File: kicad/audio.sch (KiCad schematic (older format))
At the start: 18 parts, among them J301 ST-214N, J302 ST-214N, J303 ST-214N, U301 AD824

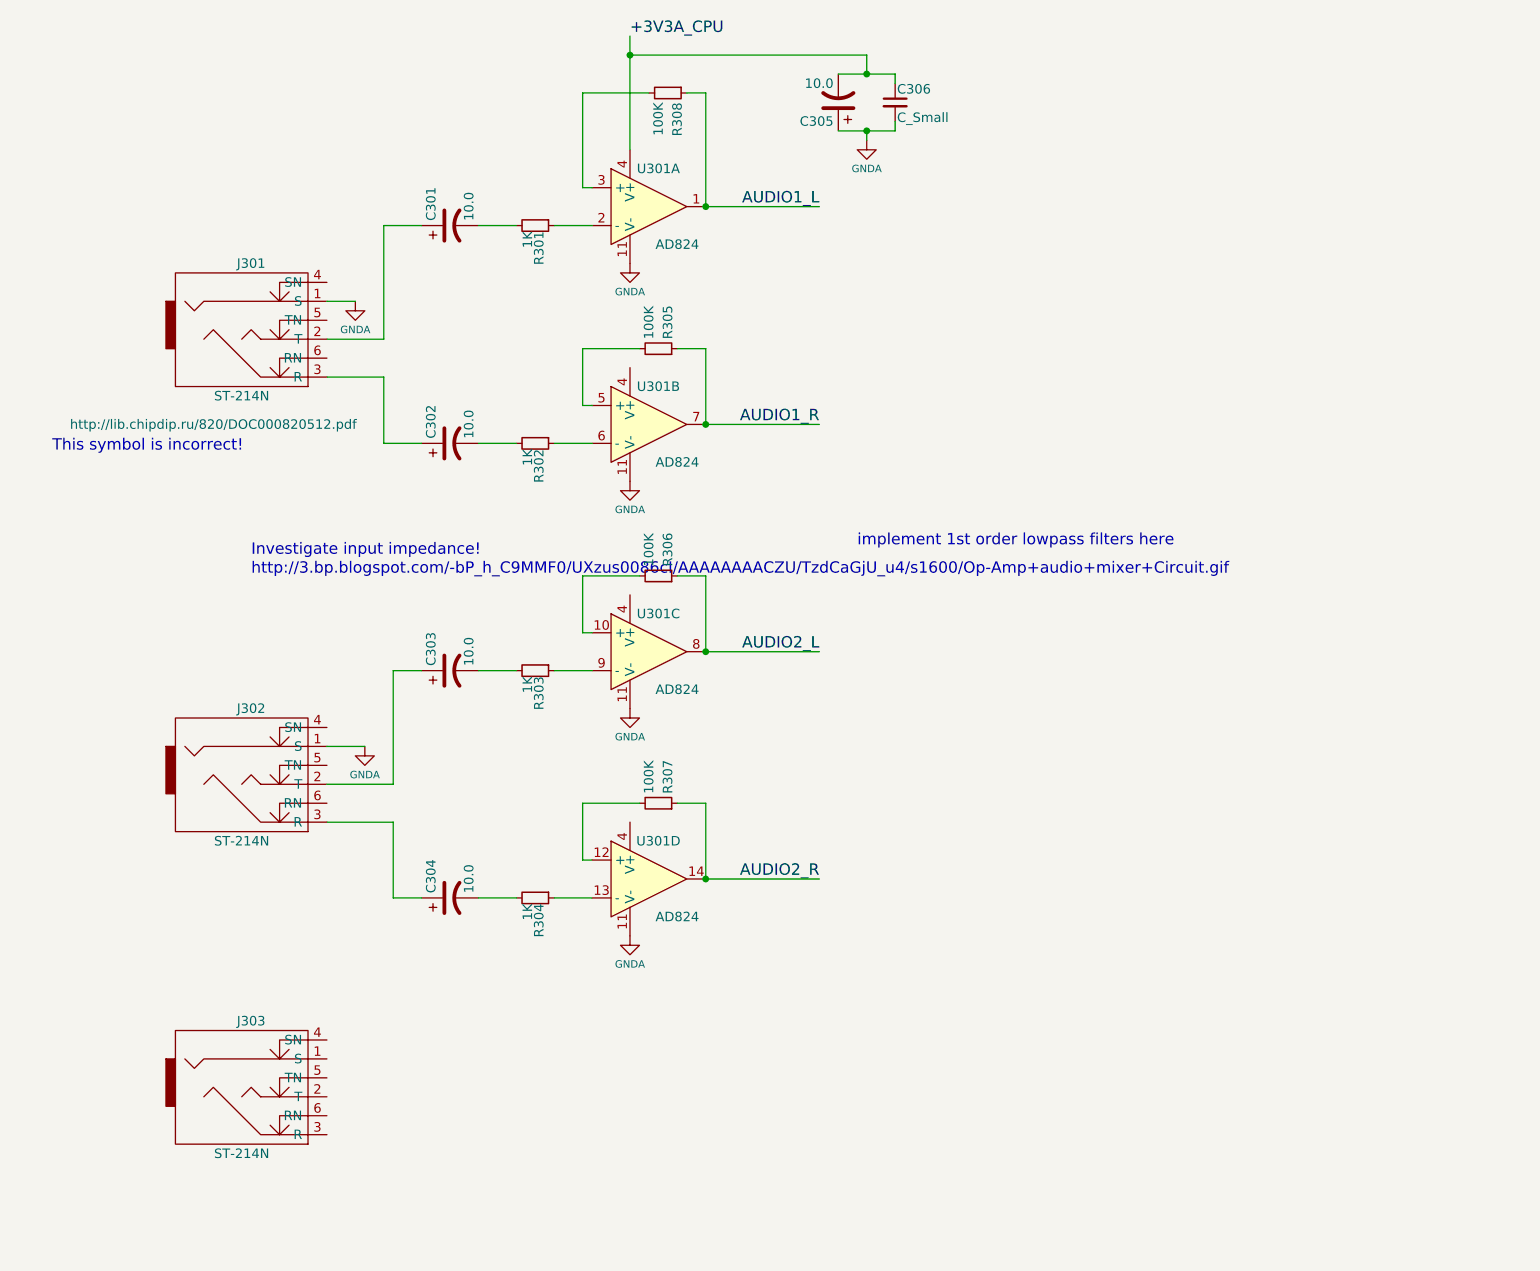
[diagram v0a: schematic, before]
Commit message: ...
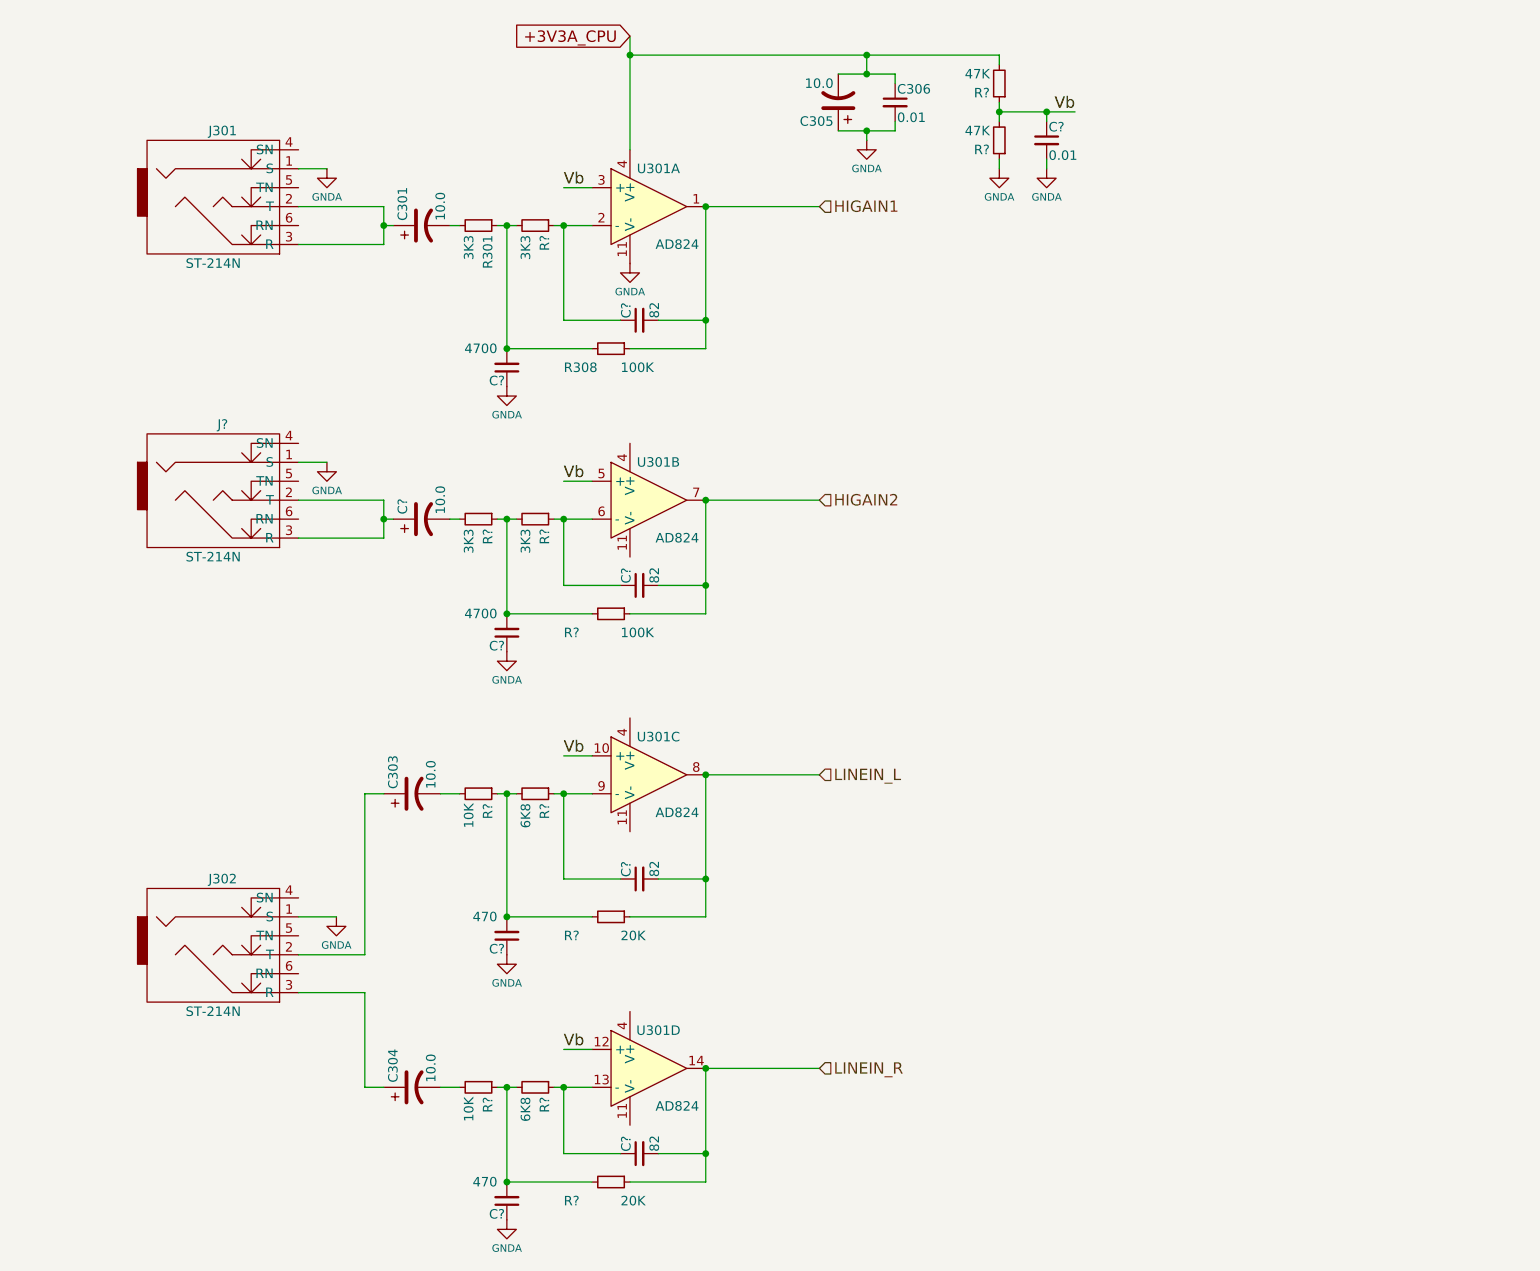
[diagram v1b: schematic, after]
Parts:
- removed C302: 10.0, symbol CP1
- removed J303: ST-214N, symbol JACK_TRS_6PINS
- removed R302, R303, R304: 1K, symbol R_Small
- removed R305, R306, R307: 100K, symbol R_Small
- added C? (x4): 82, symbol C_Small
- added C? (x2): 4700, symbol C_Small
- added C?: 0.01, symbol C_Small
- added C?: 10.0, symbol CP1
- added C? (x2): 470, symbol C_Small
- added J?: ST-214N, symbol JACK_TRS_6PINS
- added R? (x3): 3K3, symbol R_Small
- added R? (x2): 47K, symbol R_Small
- added R?: 100K, symbol R_Small
- added R? (x2): 10K, symbol R_Small
- added R? (x2): 20K, symbol R_Small
- added R? (x2): 6K8, symbol R_Small
- C306: value C_Small -> 0.01
- R301: value 1K -> 3K3
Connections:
- net +3V3A_CPU: now also R?.2
- net GNDA: now also C?.1, C?.1, C?.1, C?.1, C?.2, J?.1 (S), R?.1; no longer U301.11 (V-), U301.11 (V-), U301.11 (V-)
- net at C301.1, J301.2 (T): now also J301.3 (R)
- net at U301.2 (-): now also C?.1, R?.1; no longer R301.1
- net at R308.2: now also R301.1, C?.2, R?.2; no longer U301.3 (+)
- net Vb: now reaches U301.5 (+)
- net Vb: now also U301.10 (+), U301.12 (+), U301.3 (+), C?.1, R?.1, R?.2
- net at U301.6 (-): now also C?.1, R?.1
- net at U301.9 (-): now also C?.1, R?.1
- net at U301.13 (-): now also C?.1, R?.1
- net at C303.2: now also R?.2
- net at C304.2: now also R?.2
- net AUDIO1_L renamed HIGAIN1
- net HIGAIN1: now also C?.2
- net AUDIO1_R renamed HIGAIN2
- net HIGAIN2: now also C?.2, R?.1
- net AUDIO2_L renamed LINEIN_L
- net LINEIN_L: now also C?.2, R?.1
- net AUDIO2_R renamed LINEIN_R
- net LINEIN_R: now also C?.2, R?.1
- new net: C?.1, J?.2 (T), J?.3 (R)
- new net: C?.2, R?.2
- new net: C?.2, R?.1, R?.2, R?.2 (x3)
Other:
- note removed: "Investigate input impedance!"
- note removed: "This symbol is incorrect!"
- note removed: "http://3.bp.blogspot.com/-bP_h_C9MMF0/UXzus0086cI/AAAAAAAACZU/TzdCaGjU_u4/s1600/Op-Amp+audio+mixer+Circuit.gif"
- note removed: "implement 1st order lowpass filters here"
- moved on the sheet: C301, C303, C304, J301, J302, R301, R308, U301B, U301C, U301D
